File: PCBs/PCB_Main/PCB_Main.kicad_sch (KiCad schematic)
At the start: 12 parts, among them J1 Conn_01x03_Pin, J10 To_Audio, J3 Light Sensor Connector, J4 USB_B_Micro, J5 LED connectors, J6 XT60-M, J7 HUB75, U8 ESP32-WROVER-E

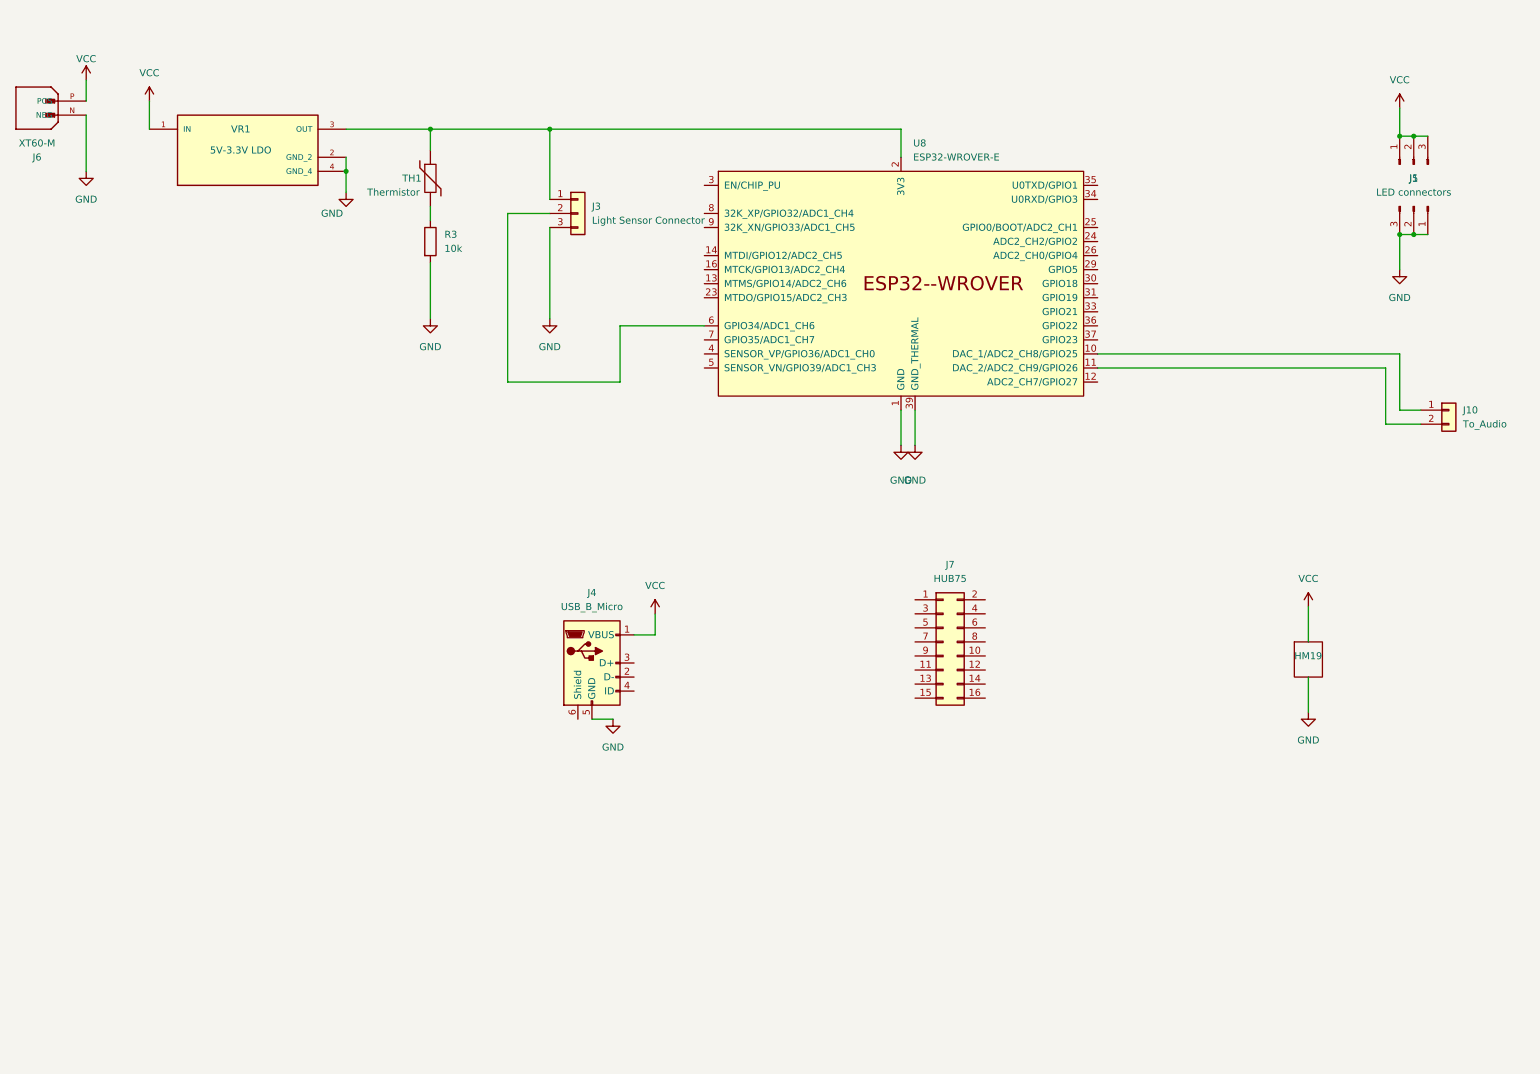
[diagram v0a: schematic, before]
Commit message: updated PCB main
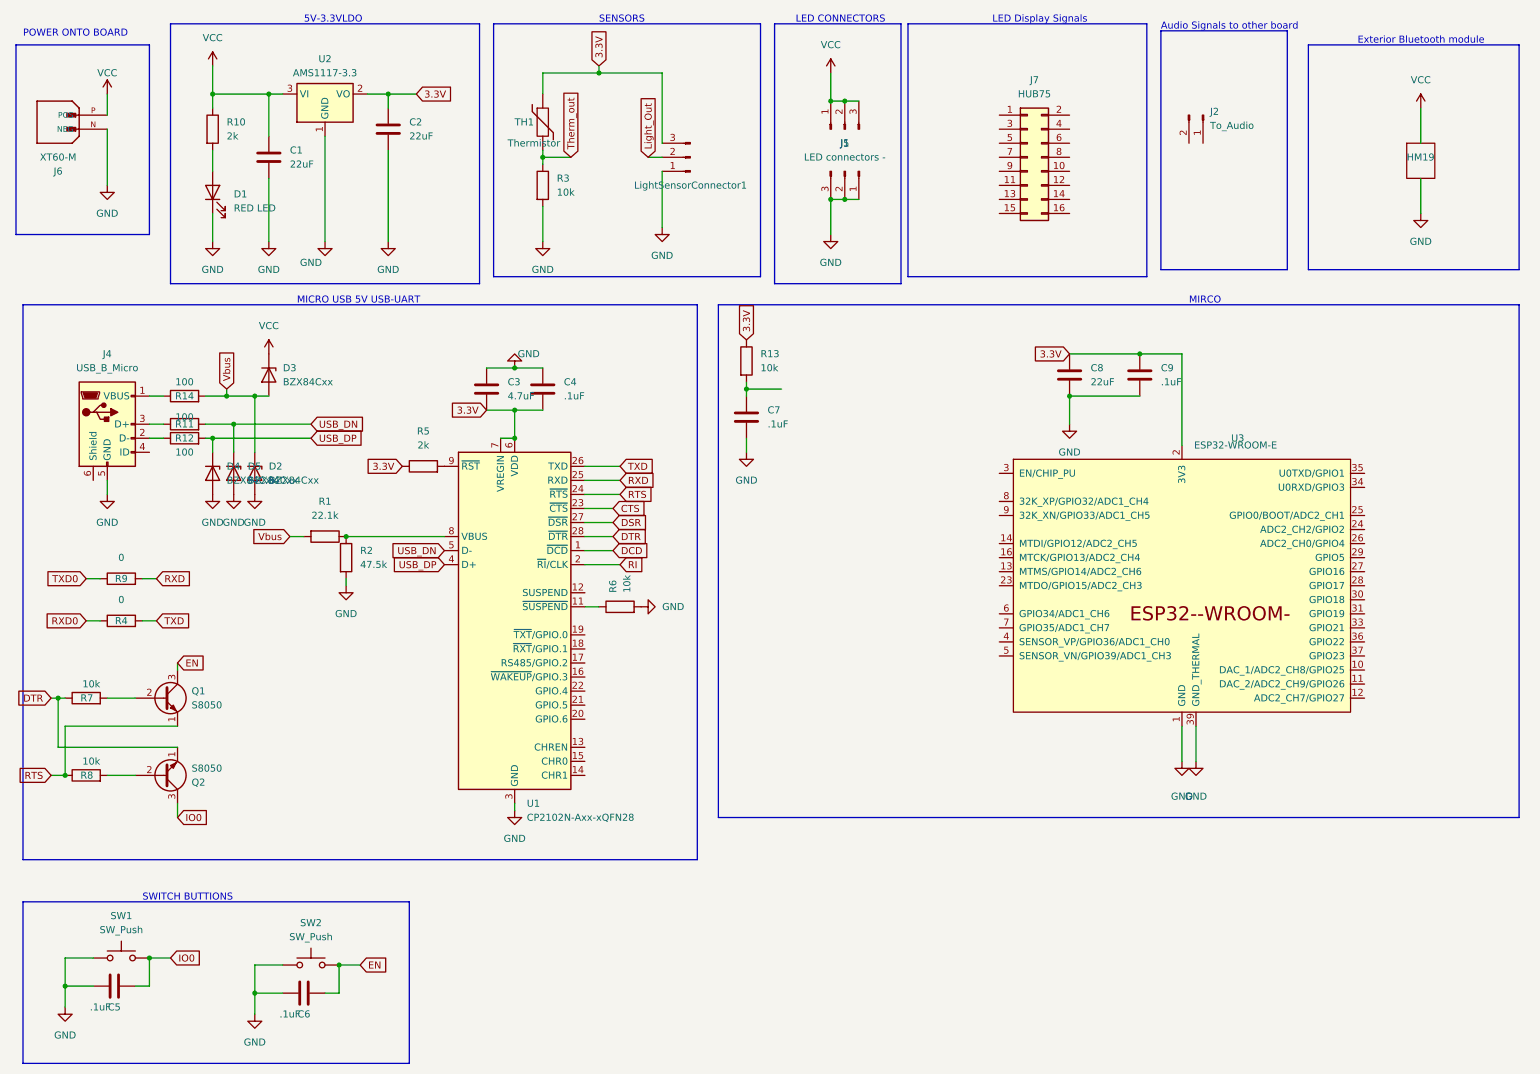
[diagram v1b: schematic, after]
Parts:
- removed J10: To_Audio, Connector_JST:JST_EH_B2B-EH-A_1x02_P2.50mm_Vertical, symbol Connector_Generic:Conn_01x02
- removed J3: Light Sensor Connector, Connector_JST:JST_EH_B3B-EH-A_1x03_P2.50mm_Vertical, symbol Connector_Generic:Conn_01x03
- removed U8: ESP32-WROVER-E, PCM_Espressif:ESP32-WROVER-E, symbol PCM_Espressif:ESP32-WROVER-E
- removed VR1: 5V-3.3V LDO, Artisyn_Components:VREG_LM3940IMP-3.3_NOPB, symbol LM3940IMP-3.3_NOPB:LM3940IMP-3.3_NOPB
- added C1, C2, C8: 22uF, Capacitor_SMD:C_0805_2012Metric, symbol Device:C
- added C3: 4.7uF, Capacitor_SMD:C_0805_2012Metric, symbol Device:C
- added C4, C5, C6, C7, C9: .1uF, Capacitor_SMD:C_0805_2012Metric, symbol Device:C
- added D1: RED LED, symbol Device:LED
- added D2, D3, D4, D5: BZX84Cxx, Package_TO_SOT_SMD:SOT-23, symbol Diode:BZX84Cxx
- added J2: To_Audio, Connector_PinHeader_2.54mm:PinHeader_1x02_P2.54mm_Vertical, symbol Connector:Conn_01x02_Pin
- added LightSensorConnector1: Conn_01x03_Pin, Connector_PinHeader_2.54mm:PinHeader_1x03_P2.54mm_Vertical, symbol Connector:Conn_01x03_Pin
- added Q1, Q2: S8050, Package_TO_SOT_THT:TO-92_Inline, symbol Transistor_BJT:S8050
- added R1: 22.1k, Resistor_SMD:R_0805_2012Metric, symbol Device:R
- added R10, R5: 2k, Resistor_SMD:R_0805_2012Metric, symbol Device:R
- added R11, R12, R14: 100, Resistor_SMD:R_0805_2012Metric, symbol Device:R
- added R13, R6, R7, R8: 10k, Resistor_SMD:R_0805_2012Metric, symbol Device:R
- added R2: 47.5k, Resistor_SMD:R_0805_2012Metric, symbol Device:R
- added R4, R9: 0, Resistor_SMD:R_0805_2012Metric, symbol Device:R
- added SW1, SW2: SW_Push, symbol Switch:SW_Push
- added U1: CP2102N-Axx-xQFN28, Package_DFN_QFN:QFN-28-1EP_5x5mm_P0.5mm_EP3.35x3.35mm, symbol Interface_USB:CP2102N-Axx-xQFN28
- added U2: AMS1117-3.3, Package_TO_SOT_SMD:SOT-223-3_TabPin2, symbol Regulator_Linear:AMS1117-3.3
- added U3: ESP32-WROOM-E, PCM_Espressif:ESP32-WROOM-32E, symbol PCM_Espressif:ESP32-WROOM-E
- J1: value Conn_01x03_Pin -> LED Connectors+
- J5: value LED connectors -> LED connectors -
- J7: footprint (none) -> Connector_PinHeader_2.54mm:PinHeader_2x08_P2.54mm_Vertical
- R3, TH1: footprint (none) -> Resistor_SMD:R_0805_2012Metric
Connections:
- net GND: now also C1.2, C2.2, C3.1, C4.1, C5.1, C6.1, C7.2, C8.2, C9.2, D1.1 (K), D2.1 (A), D4.1 (A), D5.1 (A), LightSensorConnector1.1 (Pin_1), R2.2, R6.2, SW1.1, SW2.1, U1.29 (GND), U1.3 (GND), U2.1 (GND), U3.1 (GND), U3.15 (GND), U3.38 (GND), U3.39 (GND_THERMAL)
- net VCC: now also C1.1, D3.3 (K), R10.1, U2.3 (VI); no longer J4.1 (VBUS)
- net 3.3V: now reaches TH1.1
- net 3.3V: now also C2.1, C3.2, C4.2, C8.1, C9.1, LightSensorConnector1.3 (Pin_3), R13.1, R5.1, U1.6 (VDD), U1.7 (VREGIN), U2.2 (VO), U3.2 (3V3)
- net Therm_out: now reaches R3.1, TH1.2
- net at J4.2 (D-): now also R12.1
- net at J4.3 (D+): now also R11.1
- new net: R1.1, R2.1, U1.8 (VBUS)
- new net: R5.2, U1.9 (~{RST})
- new net: R6.1, U1.11 (~{SUSPEND})
- new net: Q2.2 (B), R8.2
- new net: D1.2 (A), R10.2
- new net: Q1.2 (B), R7.2
- new net: J4.1 (VBUS), R14.1
- new net: C7.1, R13.2
- new net CTS: U1.23 (~{CTS})
- new net DCD: U1.1 (~{DCD})
- new net DSR: U1.27 (~{DSR})
- new net DTR: Q2.1 (E), R7.1, U1.28 (~{DTR})
- new net EN: C6.2, Q1.3 (C), SW2.2
- new net IO0: C5.2, Q2.3 (C), SW1.2
- new net Light_Out: LightSensorConnector1.2 (Pin_2)
- new net RI: U1.2 (~{RI}/CLK)
- new net RTS: Q1.1 (E), R8.1, U1.24 (~{RTS})
- new net RXD: R9.2, U1.25 (RXD)
- new net RXD0: R4.1
- new net TXD: R4.2, U1.26 (TXD)
- new net TXD0: R9.1
- new net USB_DN: D5.3 (K), R11.2, U1.5 (D-)
- new net USB_DP: D4.3 (K), R12.2, U1.4 (D+)
- new net Vbus: D2.3 (K), D3.1 (A), R1.2, R14.2
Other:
- note added: "5V-3.3VLDO"
- note added: "Audio Signals to other board"
- note added: "Exterior Bluetooth module"
- note added: "LED CONNECTORS"
- note added: "LED Display Signals"
- note added: "MICRO USB 5V USB-UART"
- note added: "MIRCO"
- note added: "POWER ONTO BOARD"
- note added: "SENSORS"
- note added: "SWITCH BUTTIONS"
- moved on the sheet: HM19, J1, J4, J5, J6, J7, R3, TH1
